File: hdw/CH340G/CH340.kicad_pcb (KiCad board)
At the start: 2 copper layers, 34.3 x 19.3 mm, 8 parts, among them J1 Conn_01x06, P1 USB_C_Plug_USB2.0, U1 CH340C

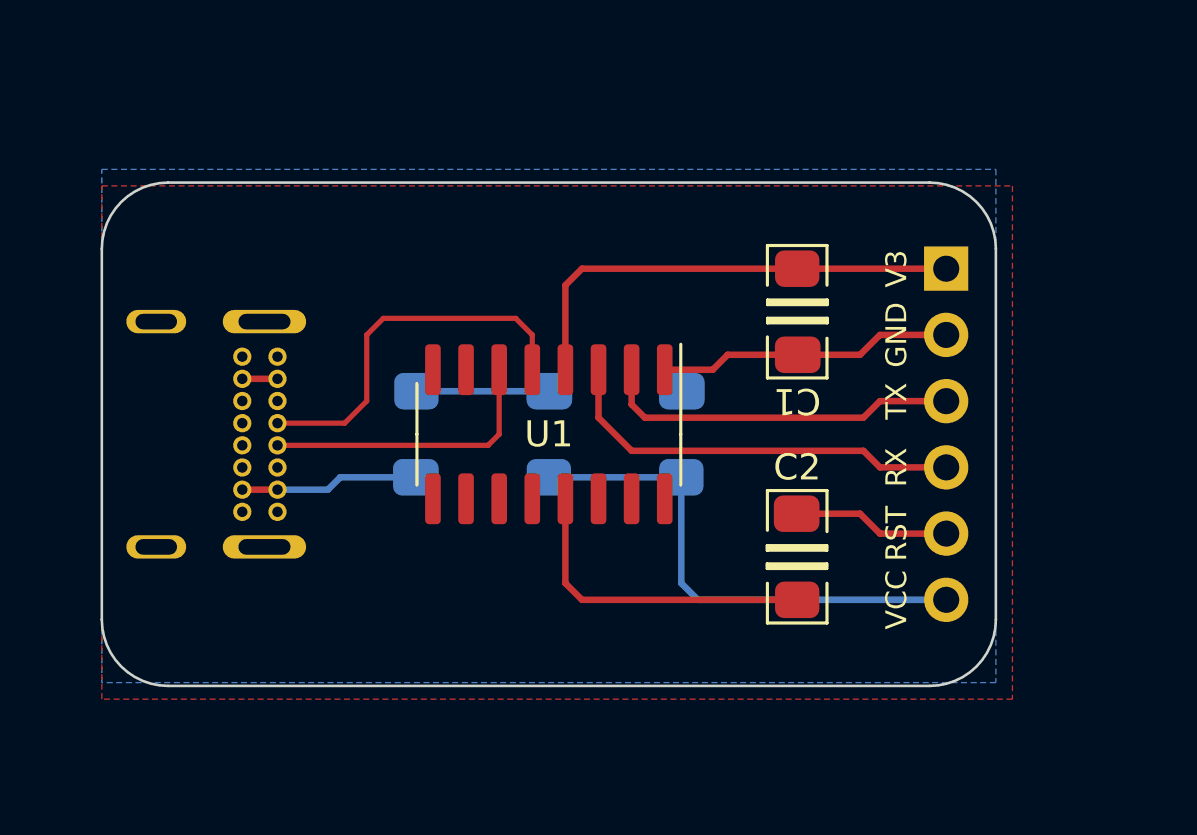
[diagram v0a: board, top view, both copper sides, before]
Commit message: wip
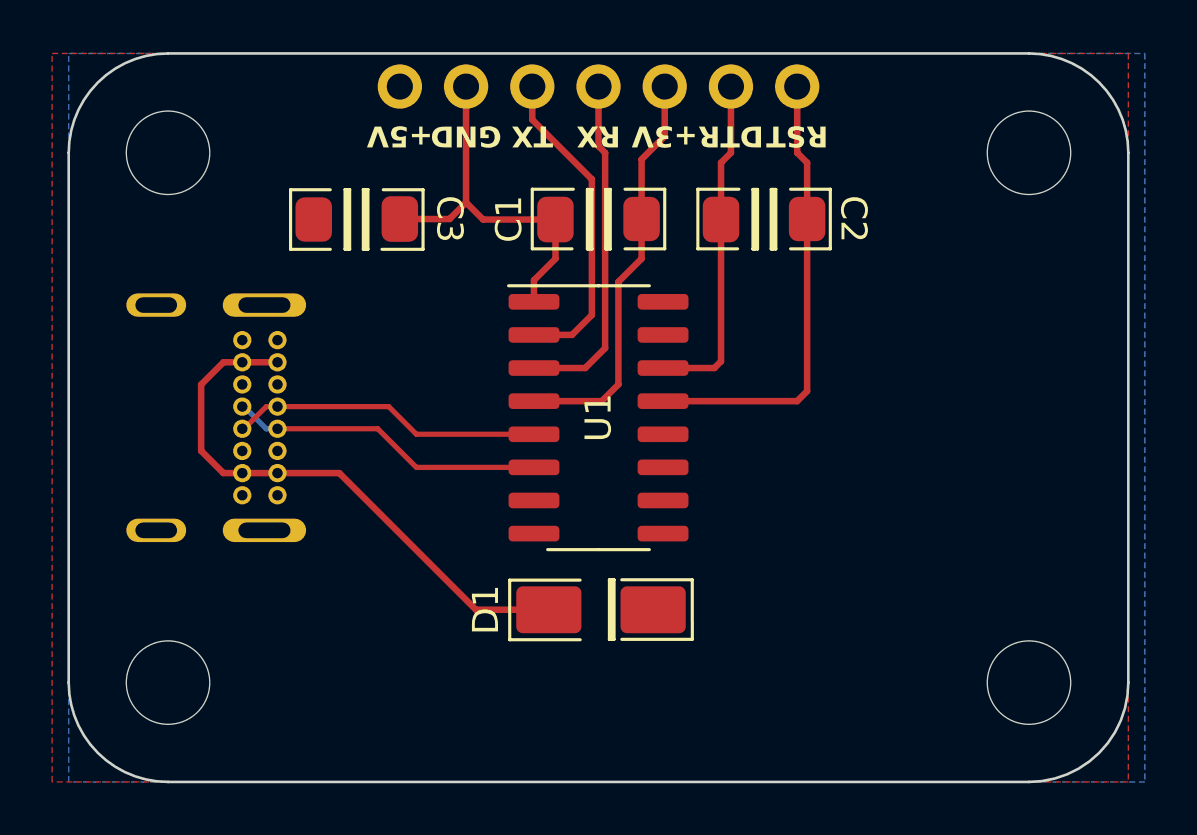
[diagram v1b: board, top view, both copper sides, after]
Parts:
- removed D3: D, Library:D1206
- removed F1: Polyfuse, Library:F1206
- added D1: D, Library:SMA_DO_214AC, F.Cu at (92.8, 120.4)
- added H1: MountingHole, MountingHole:MountingHole_3.2mm_M3, F.Cu at (76.2, 102.9)
- added H2: MountingHole, MountingHole:MountingHole_3.2mm_M3, F.Cu at (109.2, 102.9)
- added H3: MountingHole, MountingHole:MountingHole_3.2mm_M3, F.Cu at (109.2, 123.2)
- added H4: MountingHole, MountingHole:MountingHole_3.2mm_M3, F.Cu at (76.2, 123.2)
- C3: renamed from C5; moved to F.Cu
- J1: value Conn_01x06 -> Conn_01x07; footprint Connector_PinHeader_2.54mm:PinHeader_1x06_P2.54mm_Vertical -> Library:PinHeader_1x07_P2.54mm
- P1: value USB_C_Plug_USB2.0 -> USB_C_Receptacle_USB2.0
- moved C3 14.9 mm to (83.4, 105.4), turned to 0 degrees
- moved C2 13.0 mm to (99.1, 105.4), turned to 180 degrees
- moved J1 9.03 mm to (100.3, 100.3), turned to -90 degrees
- moved C1 8.41 mm to (92.7, 105.4), turned to 180 degrees
- moved U1 2.01 mm to (92.7, 113.0), turned to 0 degrees
- moved P1 0.64 mm to (76.8, 113.0)
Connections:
- C2 pad 2: RST -> RTS
- J1 pad 1: V3 -> DTR
- J1 pad 2: GND -> RTS
- J1 pad 3: TX -> V3
- J1 pad 5: RST -> TX
- J1 pad 6: VCC -> GND
- P1 pad A8: (no net) -> unconnected-(P1-SBU1-PadA8)
- P1 pad B6: (no net) -> D+
- P1 pad B7: (no net) -> D-
- P1 pad B8: (no net) -> unconnected-(P1-SBU2-PadB8)
- P1 pad S1: unconnected-(P1-SHIELD-PadS1) -> GND
- U1 pad 14: unconnected-(U1-~{RTS}-Pad14) -> RTS
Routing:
- net VCC: track 19.6 -> 0.00 mm
- net VBUS: track 8.20 -> 21.6 mm
- net RTS: track 0.00 -> 13.0 mm
- net RST: track 6.05 -> 0.00 mm
- net DTR: track 12.4 -> 17.5 mm
- net Net-(D3-K): track 5.10 -> 0.00 mm
- net GND: track 11.3 -> 14.4 mm
- net RX: track 16.0 -> 13.2 mm
- net D+: track 14.5 -> 12.0 mm
- net V3: track 18.1 -> 15.7 mm
- net TX: track 13.9 -> 12.2 mm
- net D-: track 11.2 -> 12.2 mm
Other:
- board size 34.3 x 19.3 mm -> 40.6 x 27.9 mm
- board text added: "+3V"
- board text added: "+5V"
- board text added: "CH340G"
- board text added: "DTR"
- board text added: "V2.2 2024-04"
- board text added: "nicola@strappazzon.me"
- board text removed: "CH340"
- board text removed: "V2 2024/01"
- board text removed: "V3"
- board text removed: "VCC"
- board text removed: "nstrappazzonc"
